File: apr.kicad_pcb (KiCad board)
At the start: 2 copper layers, 198.5 x 154 mm, 94 parts, among them J1 Screw_Terminal_01x03, J10 Screw_Terminal_01x02, J11 Screw_Terminal_01x02, J12 Screw_Terminal_01x02, J13 Conn_01x04, J14 Conn_01x04, J15 Flash Module Conn, J16 Bateria Lítio 1, J17 Bateria Lítio 2, J18 LORA, J19 LORA, J2 Screw_Terminal_01x03, J20 Screw_Terminal_01x02, J21 Screw_Terminal_01x02, J22 Screw_Terminal_01x02, J23 Conn_01x20_Pin, J24 Conn_01x20_Pin, J25 Screw_Terminal_01x02, J26 Screw_Terminal_01x02, J27 Screw_Terminal_01x02, J28 Screw_Terminal_01x02, J29 A1, J3 Screw_Terminal_01x02, J30 Screw_Terminal_01x03, J31 Bateria Lítio 3, J32 Buzzer, J33 Bateria Lipo, J34 A2, J35 11, J36 12, J37 14, J4 Screw_Terminal_01x02, J5 Screw_Terminal_01x02, J6 Conn_01x20_Pin, J7 Conn_01x20_Pin, J8 Screw_Terminal_01x02, J9 Screw_Terminal_01x02, Q10 IRLZ34N, Q11 IRLZ34N, Q2 IRLZ34N, Q3 IRLZ34N, Q4 IRLZ34N, Q5 IRLZ34N, Q6 IRLZ34N, Q7 IRLZ34N, Q8 IRLZ34N, Q9 IRLZ34N, U3 LM7905_TO220

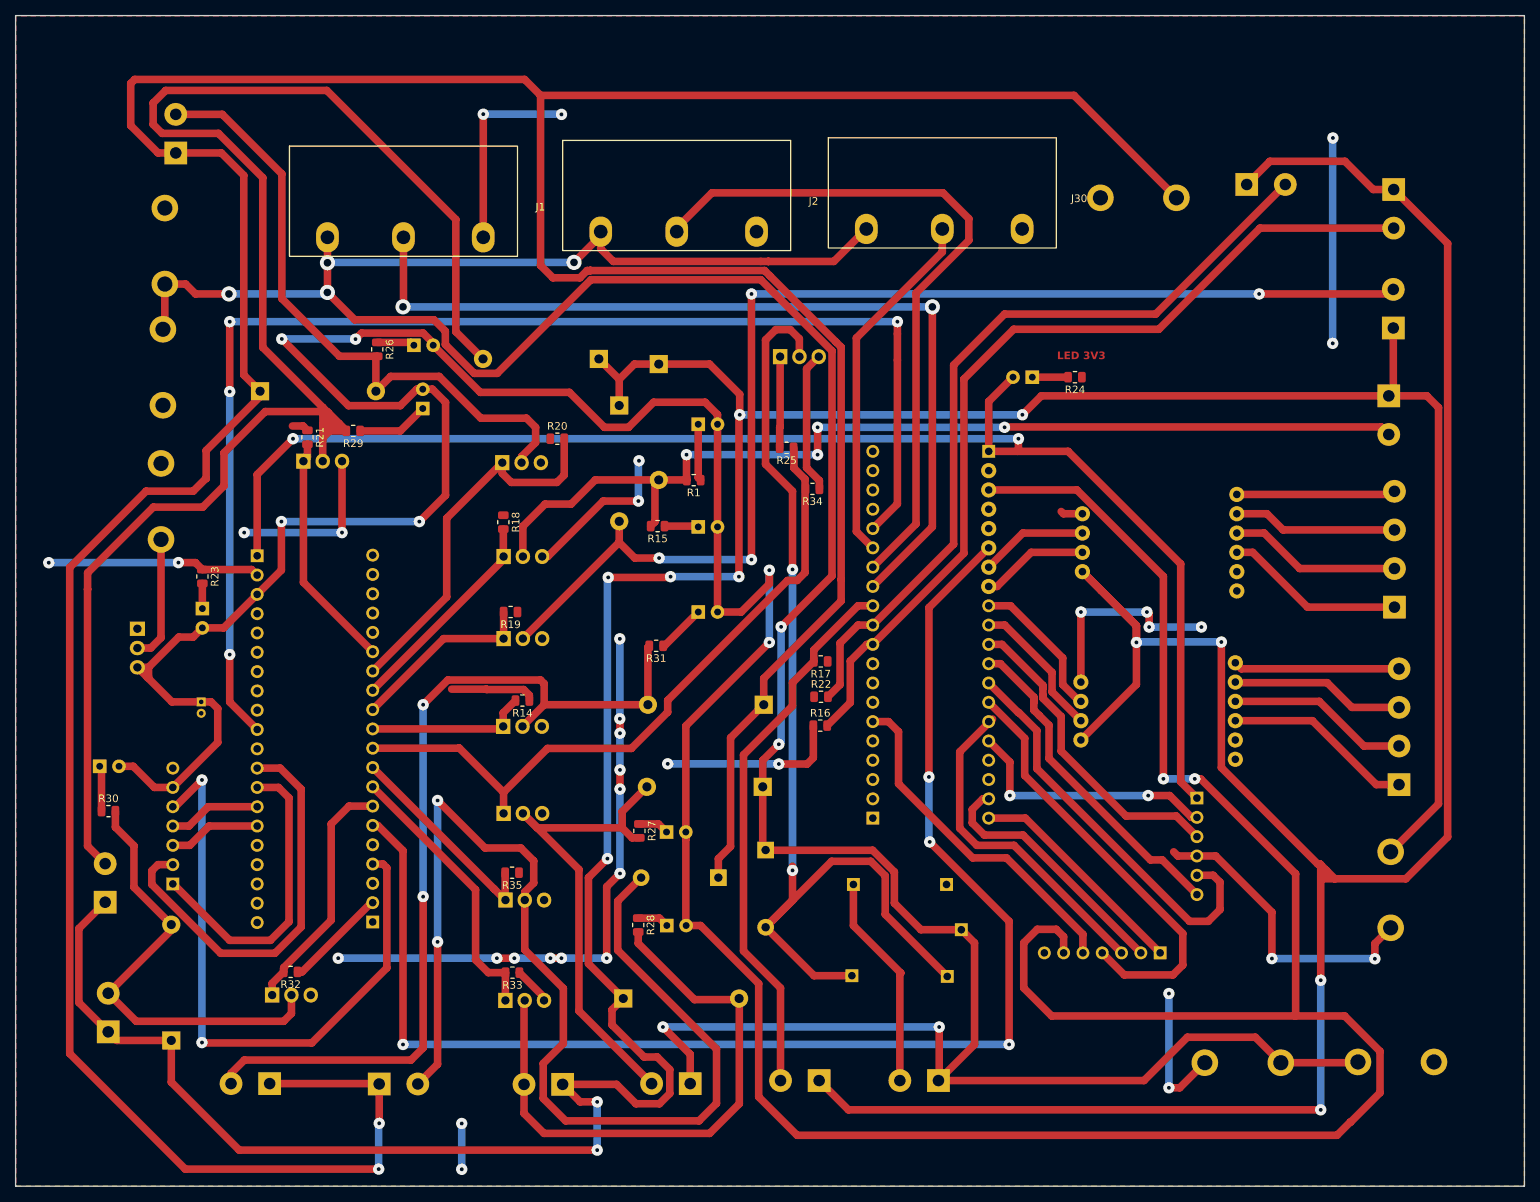
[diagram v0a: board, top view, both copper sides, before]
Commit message: Esquemático e Layout PCB Sólido
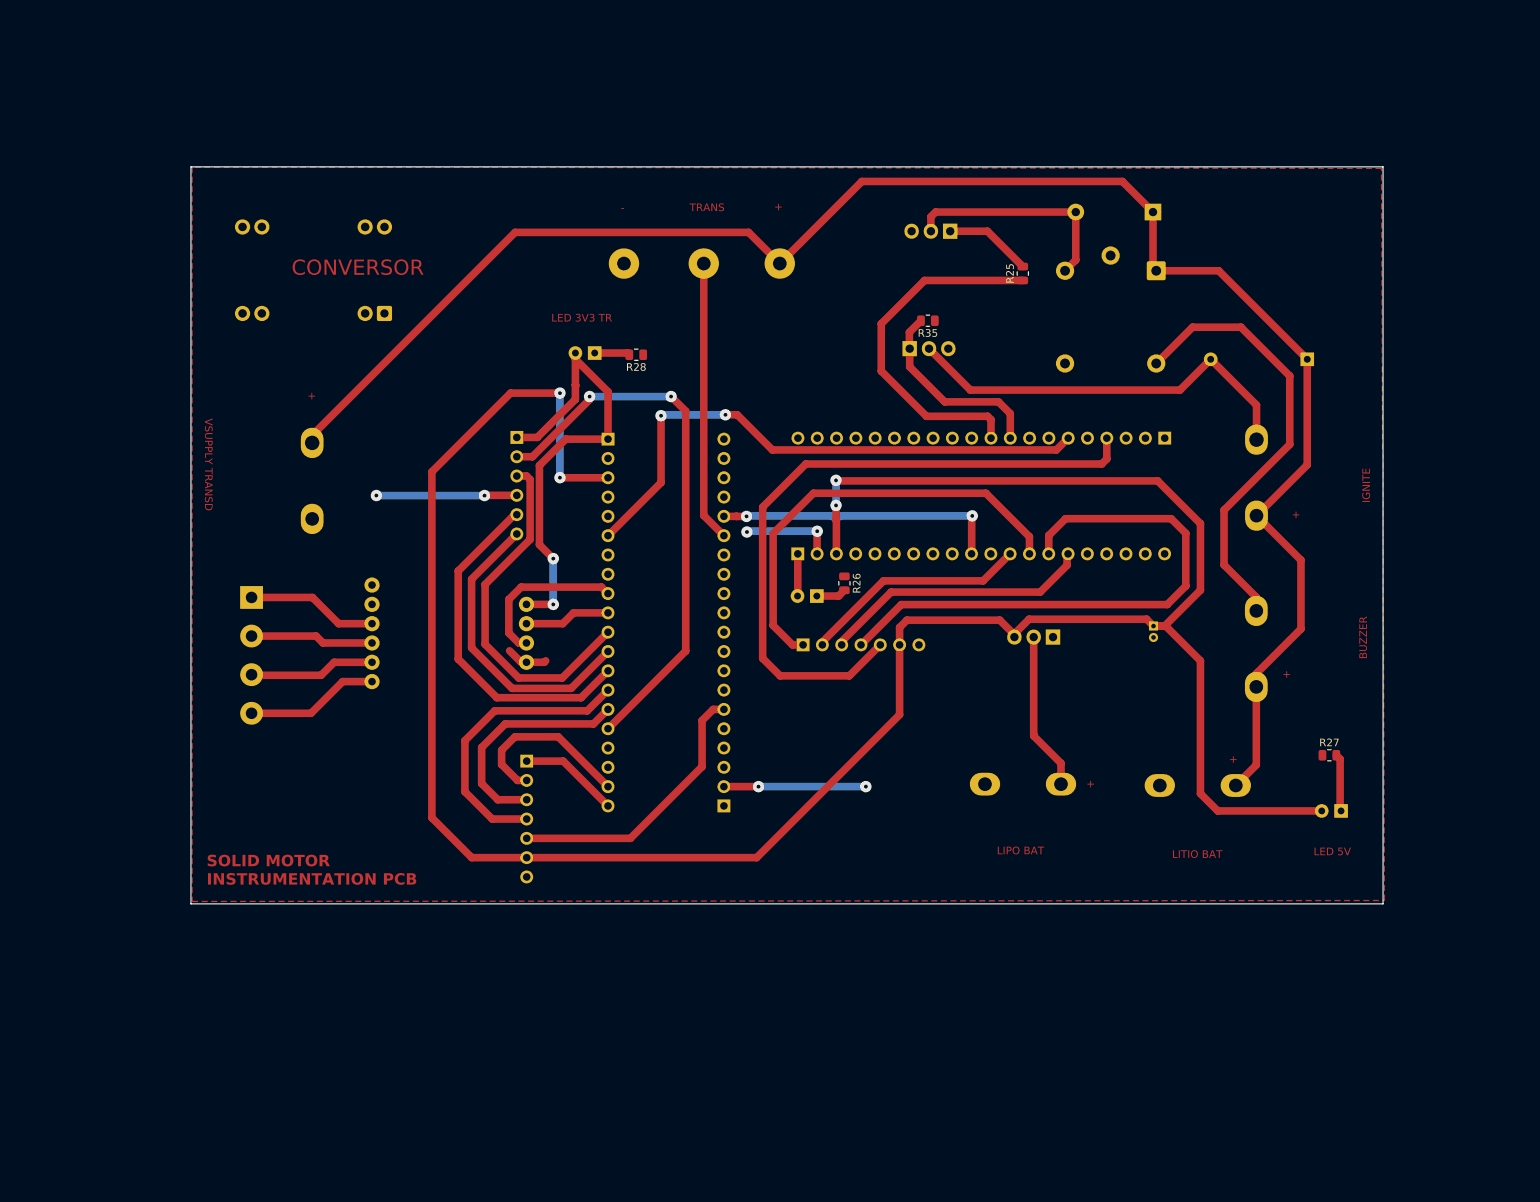
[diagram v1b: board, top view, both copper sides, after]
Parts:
- removed CR2, CR3, CR4, CR5, CR6, CR7, CR8: UF4007-E3/73, Diode_THT:D_DO-15_P15.24mm_Horizontal
- removed D1: 1N4007, Diode_THT:D_DO-41_SOD81_P10.16mm_Horizontal
- removed D10, D17, D18, D19, D2, D20, D3: LED, LED_THT:LED_D5.0mm
- removed J1, J2: Screw_Terminal_01x03, Library:KT100-3PIN
- removed J10, J11, J12, J20, J21, J22, J3, J4, J5, J8, J9: Screw_Terminal_01x02, TerminalBlock:TerminalBlock_bornier-2_P5.08mm
- removed J14: Conn_01x04, TerminalBlock:TerminalBlock_bornier-4_P5.08mm
- removed J16: Bateria Lítio 1, Library:Screw Terminal 3D
- removed J17: Bateria Lítio 2, Library:Screw Terminal 3D
- removed J27, J28: Screw_Terminal_01x02, Library:Screw Terminal 3D
- removed J29: A1, Connector_PinHeader_2.54mm:PinHeader_1x01_P2.54mm_Vertical
- removed J34: A2, Connector_PinHeader_2.54mm:PinHeader_1x01_P2.54mm_Vertical
- removed J35: 11, Connector_PinHeader_2.54mm:PinHeader_1x01_P2.54mm_Vertical
- removed J36: 12, Connector_PinHeader_2.54mm:PinHeader_1x01_P2.54mm_Vertical
- removed J37: 14, Connector_PinHeader_2.54mm:PinHeader_1x01_P2.54mm_Vertical
- removed Q2, Q3, Q4, Q5, Q6, Q7, Q8, Q9: IRLZ34N, Package_TO_SOT_THT:TO-220-3_Vertical
- removed R1, R15, R23, R24, R29, R30, R31: 470, Resistor_SMD:R_0805_2012Metric
- removed R14, R18, R19, R20, R21, R32, R33, R34: 4K7, Resistor_SMD:R_0805_2012Metric
- removed R16: 5.6k, Resistor_SMD:R_0805_2012Metric
- removed R17: 270k, Resistor_SMD:R_0805_2012Metric
- removed R22: 390k, Resistor_SMD:R_0805_2012Metric
- added K1: Fujitsu_FTR-LYCA005x, Relay_THT:Relay_SPDT_Finder_36.11, B.Cu at (208.9, 51.1)
- CR1: footprint Diode_THT:D_DO-15_P15.24mm_Horizontal -> Diode_THT:D_A-405_P12.70mm_Horizontal
- J25: value Screw_Terminal_01x02 -> VSUPPLY TRANSDUCER
- J26: value Screw_Terminal_01x02 -> IGNITION; footprint TerminalBlock:TerminalBlock_bornier-2_P5.08mm -> Library:Screw Terminal 3D
- J30: moved to B.Cu
- J31: value Bateria Lítio 3 -> Bateria Lítio
- J32: footprint TerminalBlock:TerminalBlock_bornier-2_P5.08mm -> Library:Screw Terminal 3D
- U1: value ~ -> Ag9905LP; footprint Library:hx711 -> Converter_DCDC:Converter_DCDC_Silvertel_Ag99xxLP_THT
- moved J25 164.0 mm to (97.8, 83.8), turned to 90 degrees
- moved J13 153.0 mm to (89.8, 94.1), turned to -90 degrees
- moved J26 137.5 mm to (222.1, 83.3), turned to 90 degrees
- moved C1 125.7 mm to (208.5, 97.8)
- moved J33 122.7 mm to (196.3, 118.7), turned to 180 degrees
- moved J6 122.1 mm to (210.0, 73.1), turned to 90 degrees
- moved U3 120.5 mm to (195.3, 99.3), turned to 180 degrees
- moved U1 114.7 mm to (107.3, 56.7), turned to 90 degrees
- moved U2 113.6 mm to (105.7, 105.2), turned to 0 degrees
- moved J15 101.3 mm to (124.7, 73.0)
- moved D4 98.2 mm to (208.4, 43.4), turned to 180 degrees
- moved D6 92.5 mm to (233.2, 122.2), turned to 180 degrees
- moved R27 91.3 mm to (231.6, 114.8), turned to 0 degrees
- moved R35 90.9 mm to (178.8, 57.7)
- moved Q10 90.0 mm to (176.4, 61.4)
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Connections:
- net /TRANSDUCER_CAMARA_PA0 renamed /TRANSDUCER
- CR1 pad 1: +12C -> +12V
- CR1 pad 2: /QUICK_DISCONNECT -> /IGNITE
- D5 pad 2: +5V -> +3.3V
- D7 pad 2: +5V -> +3V3
- J23 pad 7: /DT2 -> unconnected-(J23-Pin_7-Pad7)
- J23 pad 8: /SCK2 -> unconnected-(J23-Pin_8-Pad8)
- J24 pad 10: /THERMISTOR_CAMARA -> unconnected-(J24-Pin_10-Pad10)
- J24 pad 11: /THERMISTOR_LINE -> unconnected-(J24-Pin_11-Pad11)
- J24 pad 12: /THERMISTOR_TANK -> unconnected-(J24-Pin_12-Pad12)
- J24 pad 13: /TRANSDUCER_LINE_PA2 -> unconnected-(J24-Pin_13-Pad13)
- J24 pad 14: /TRANSDUCER_TANK_PA1 -> unconnected-(J24-Pin_14-Pad14)
- J26 pad 1: +12C -> +12V
- J6 pad 11: /QUICK_DISCONNECT_PA4 -> unconnected-(J6-Pin_11-Pad11)
- J6 pad 12: /SUPER_CHARGE_PA3 -> unconnected-(J6-Pin_12-Pad12)
- J6 pad 13: /PURGE_LINE_PA2 -> unconnected-(J6-Pin_13-Pad13)
- J6 pad 14: /VENT_PA1 -> unconnected-(J6-Pin_14-Pad14)
- J6 pad 15: /FUEL_LINE_A0 -> unconnected-(J6-Pin_15-Pad15)
- J6 pad 7: /PURGE_TANK_PB0 -> unconnected-(J6-Pin_7-Pad7)
- J6 pad 8: /INJECTION_PA7 -> unconnected-(J6-Pin_8-Pad8)
- J7 pad 1: +3V3 -> +3.3V
- R26 pad 1: Net-(D7-K) -> GND
- R26 pad 2: /VENT -> Net-(D5-K)
- R27 pad 1: Net-(D10-K) -> GND
- R27 pad 2: /ARM -> Net-(D6-K)
- R28 pad 1: Net-(D17-K) -> GND
- R28 pad 2: /INJECTION -> Net-(D7-K)
- U1 pad 1: Net-(J14-Pin_4) -> unconnected-(U1-+VDC-Pad1)_1
- U1 pad 2: Net-(J14-Pin_3) -> unconnected-(U1-+VDC-Pad1)
- U1 pad 3: Net-(J14-Pin_2) -> unconnected-(U1--VDC-Pad3)
- U1 pad 4: Net-(J14-Pin_1) -> unconnected-(U1-ADJ-Pad4)
- U1 pad 7: +3.3V -> unconnected-(U1-VIN--Pad7)_1
- U1 pad 8: /SCK2 -> unconnected-(U1-VIN--Pad7)
- U2 pad 7: +3.3V -> +3V3
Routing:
- net +12C: track 514.3 -> 0.00 mm, vias 2 -> 0
- net +12L: track 428.1 -> 0.00 mm, vias 8 -> 0
- net GND: track 373.0 -> 54.9 mm, vias 34 -> 6
- net +3.3V: track 319.5 -> 5.56 mm, vias 4 -> 0
- net +5V: track 561.1 -> 322.9 mm, vias 8 -> 4
- net /FUEL_LINE: track 225.6 -> 0.00 mm
- net +12V: track 429.8 -> 228.5 mm, vias 8 -> 0
- net /SUPER_CHARGE: track 158.7 -> 0.00 mm, vias 4 -> 0
- net /PURGE_LINE: track 134.4 -> 0.00 mm, vias 4 -> 0
- net /RESET_PB3: track 171.6 -> 37.8 mm, vias 4 -> 2
- net +3V3: track 189.0 -> 62.1 mm
- net /QUICK_DISCONNECT: track 119.0 -> 0.00 mm, vias 2 -> 0
- net /TRANSDUCER_LINE_PA2: track 118.9 -> 0.00 mm, vias 2 -> 0
- net /THERMISTOR_CAMARA: track 118.3 -> 0.00 mm
- net Net-(D4-A): track 144.4 -> 29.5 mm, vias 2 -> 0
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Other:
- board size 198.5 x 154 mm -> 156.8 x 97 mm
- board text added: "+"
- board text added: "-"
- board text added: "BUZZER"
- board text added: "CONVERSOR"
- board text added: "IGNITE"
- board text added: "LED 3V3 TR"
- board text added: "LED 5V"
- board text added: "LIPO BAT"
- board text added: "LITIO BAT"
- board text added: "SOLID MOTOR INSTRUMENTATION PCB"
- board text added: "TRANS"
- board text added: "VSUPPLY TRANSD"
- board text removed: "LED 3V3"

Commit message: Layout Final
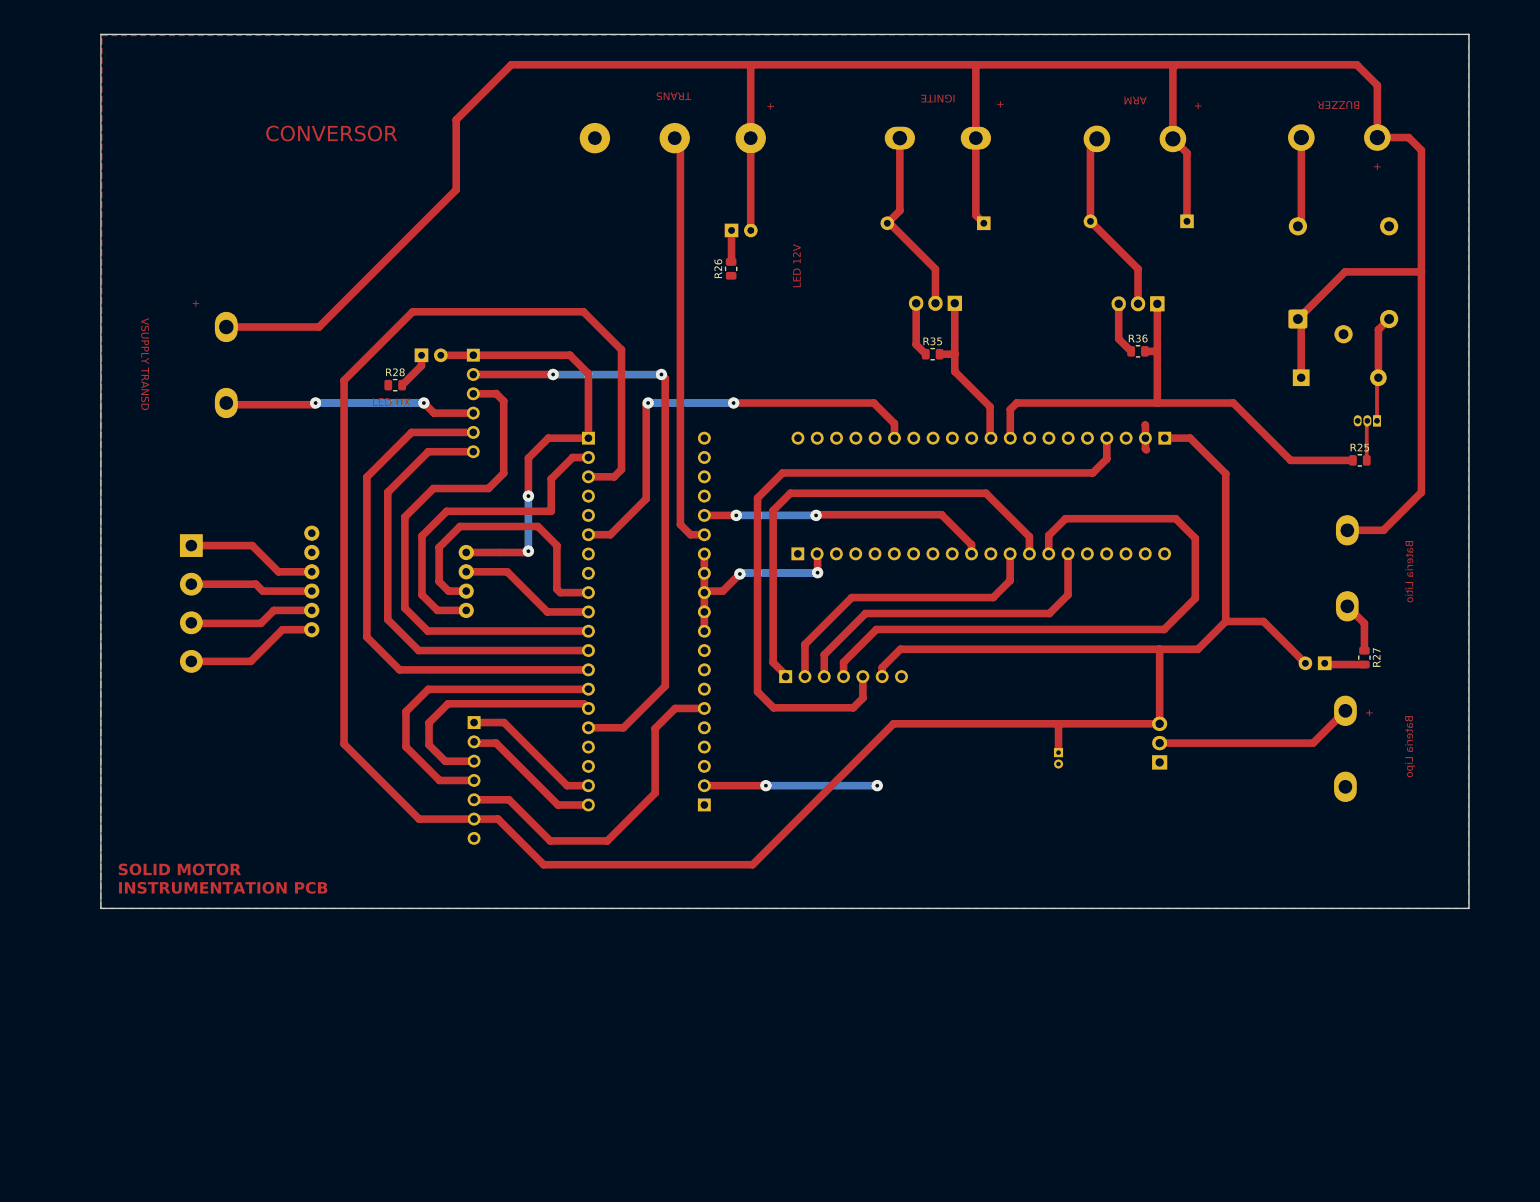
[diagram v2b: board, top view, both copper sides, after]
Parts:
- removed Q11: IRLZ34N, Package_TO_SOT_THT:TO-220-3_Vertical
- removed U1: Ag9905LP, Converter_DCDC:Converter_DCDC_Silvertel_Ag99xxLP_THT
- added CR2: UF4007-E3/73, Diode_THT:D_A-405_P12.70mm_Horizontal, B.Cu at (212.9, 44.6)
- added J27: ARM, Library:Screw Terminal 3D, B.Cu at (211.1, 33.8)
- added Q1: BC547, Package_TO_SOT_THT:TO-92_Inline, B.Cu at (237.9, 70.8)
- added Q12: IRLZ34N, Package_TO_SOT_THT:TO-220-3_Vertical, B.Cu at (209.0, 55.5)
- added R36: 4K7, Resistor_SMD:R_0805_2012Metric, F.Cu at (206.5, 61.7)
- moved J32 74.0 mm to (237.9, 33.6), turned to 180 degrees
- moved J26 61.9 mm to (185.1, 33.6), turned to 180 degrees
- moved R25 50.7 mm to (235.6, 76.0), turned to 0 degrees
- moved D5 49.4 mm to (153.0, 45.8), turned to 0 degrees
- moved CR1 46.2 mm to (186.2, 44.9)
- moved R26 44.0 mm to (152.9, 50.9), turned to 90 degrees
- moved J33 38.6 mm to (233.8, 109.0), turned to -90 degrees
- moved J31 34.1 mm to (234.0, 95.2), turned to 90 degrees
- moved R28 32.0 mm to (108.7, 66.2), turned to 0 degrees
- moved D4 29.2 mm to (227.9, 65.2), turned to 0 degrees
- moved D7 22.8 mm to (112.2, 62.2), turned to 0 degrees
- moved U3 21.7 mm to (209.3, 115.8), turned to 90 degrees
- moved C1 20.8 mm to (196.0, 114.5)
- moved K1 19.7 mm to (227.5, 57.5), turned to 0 degrees
- moved D6 19.5 mm to (231.0, 102.8)
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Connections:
- D5 pad 2: +3.3V -> +12V
- J19 pad 1: /M0_PB12 -> /M0_PB13
- J19 pad 2: /M1_PB13 -> /M1_PB12
- J23 pad 19: /M1_PB13 -> /M0_PB13
- J23 pad 20: /M0_PB12 -> /M1_PB12
- J23 pad 6: /SAVE_PB1 -> /SAVE_PA1
- J24 pad 10: unconnected-(J24-Pin_10-Pad10) -> GND
- J24 pad 11: unconnected-(J24-Pin_11-Pad11) -> GND
- J24 pad 12: unconnected-(J24-Pin_12-Pad12) -> GND
- J24 pad 13: unconnected-(J24-Pin_13-Pad13) -> GND
- J24 pad 14: unconnected-(J24-Pin_14-Pad14) -> GND
- J6 pad 1: unconnected-(J6-Pin_1-Pad1) -> +5V
- J6 pad 10: /ARM_PA5 -> /IGINTE_PA5
- J6 pad 15: unconnected-(J6-Pin_15-Pad15) -> /SAVE_PA1
- J6 pad 6: /SAVE_PB1 -> unconnected-(J6-Pin_6-Pad6)
- J6 pad 9: /IGNITE_PA6 -> /ARM_PA6
- J7 pad 3: +5V -> unconnected-(J7-Pin_3-Pad3)
- Q10 pad 1: /IGNITE_PA6 -> /IGINTE_PA5
- R25 pad 1: /ARM_PA5 -> /ARM_PA6
- R35 pad 2: /IGNITE_PA6 -> /IGINTE_PA5
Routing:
- net +12V: track 228.5 -> 334.1 mm
- net GND: track 54.9 -> 152.6 mm
- net /SAVE_PB1: track 74.9 -> 0.00 mm, vias 2 -> 0
- net /ARM_PA6: track 0.00 -> 67.1 mm
- net /SAVE_PA1: track 0.00 -> 57.7 mm, vias 0 -> 2
- net /ARM_PA5: track 46.7 -> 0.00 mm
- net Net-(J32-Pin_2): track 58.5 -> 11.9 mm
- net /IGNITE: track 54.1 -> 25.5 mm
- net /IGNITE_PA6: track 25.7 -> 0.00 mm
- net /ARM: track 0.00 -> 24.6 mm
- net /M1_PB13: track 23.5 -> 0.00 mm
- net /FLASH_SCK: track 45.6 -> 68.4 mm
- net /IGINTE_PA5: track 0.00 -> 21.7 mm
- net /FLASH_MISO: track 46.6 -> 66.7 mm
- net /FLASH_MOSI: track 39.6 -> 58.3 mm
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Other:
- board size 156.8 x 97 mm -> 180 x 115 mm
- board text added: "ARM"
- board text added: "LED 12V"
- board text added: "LED HX"
- board text removed: "-"
- board text removed: "LED 3V3 TR"
- board text removed: "LED 5V"
- board text removed: "LIPO BAT"
- board text removed: "LITIO BAT"
